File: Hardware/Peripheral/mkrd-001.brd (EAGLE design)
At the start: 25 x 26 mm, 5 parts, among them J1 MKR

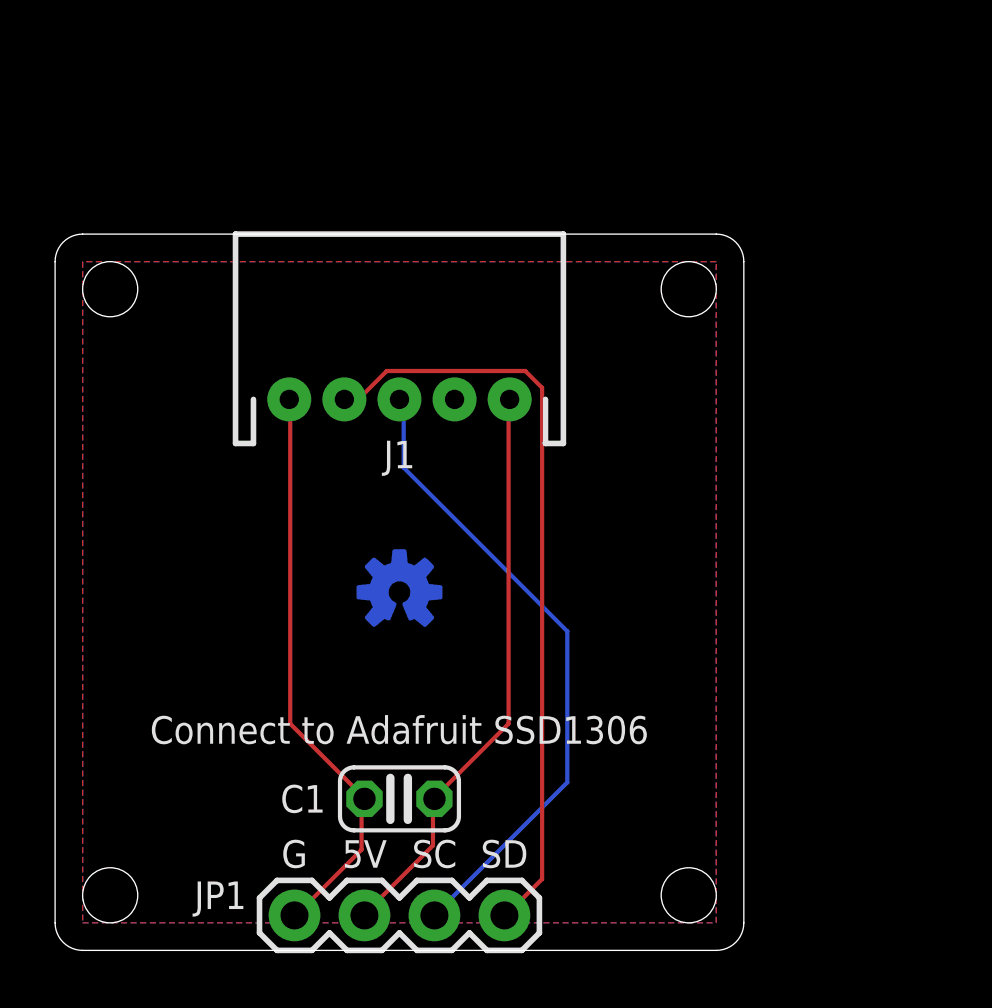
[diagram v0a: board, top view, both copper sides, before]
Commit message: Added new board.
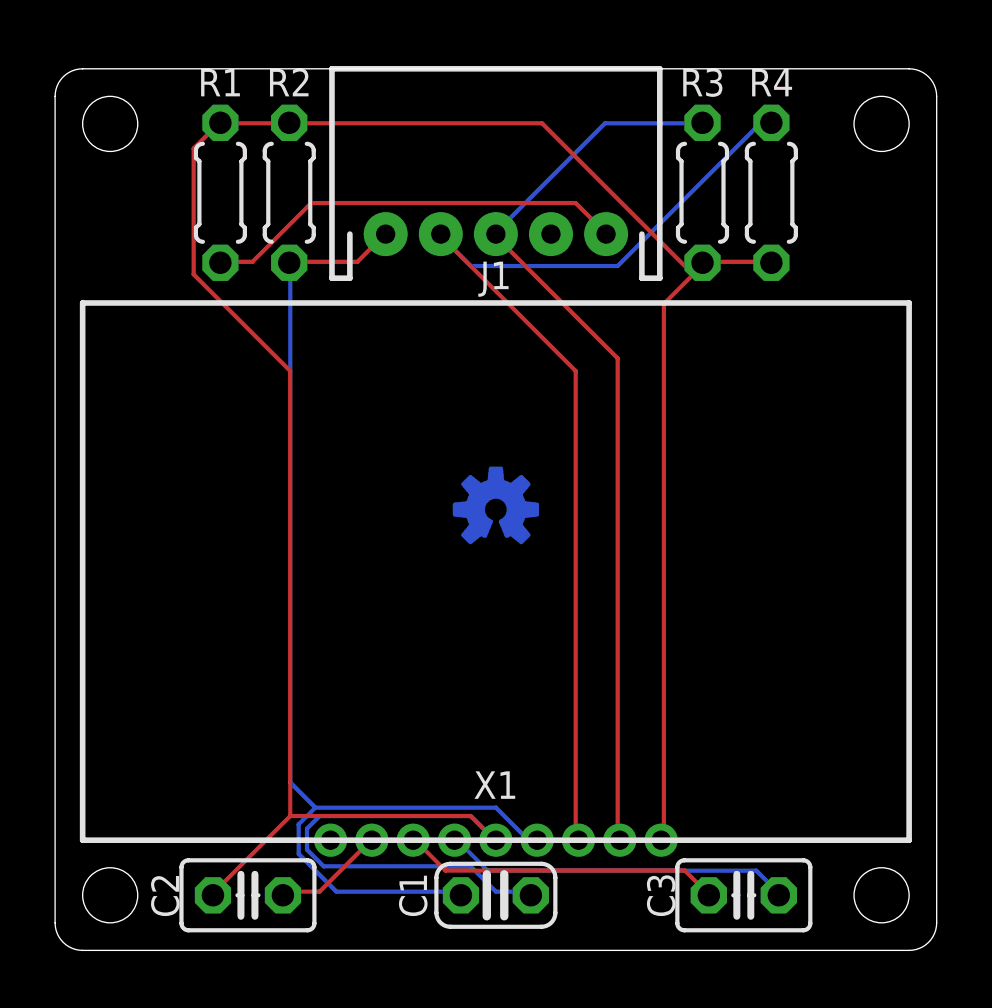
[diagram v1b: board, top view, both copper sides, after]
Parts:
- removed JP1: DISP, SparkFun-Connectors:1X04
- added C2, C3: 1u, rcl:C025-025X050
- added R1: 1.5k, rcl:0204/5
- added R2: 3.3k, rcl:0204/5
- added R3, R4: 10k, rcl:0204/5
- added X1: AQM0802A-RN-GBW, AQM0802A-RN-GBW:AQM0802A-RN-GBW-FOOTPRINT
- C1: value (none) -> 0.1u
- moved J1 6.95 mm to (16.0, 26.0)
- moved C1 4.95 mm to (16.0, 2.00)
- moved LOGO1 4.61 mm to (16.0, 16.0)
- moved U$1 4.61 mm to (16.0, 10.0)
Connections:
- new net 3V3: C1.1, C2.1, R1.2, R2.2, R3.1, R4.1, X1.5, X1.9
- new net N$1: C2.2, X1.2
- new net N$2: C3.2, X1.4
- new net N$3: C3.1, X1.3
- net GND: now also R2.1, X1.6; no longer JP1.1
- net SCL: now also R3.2, X1.8; no longer JP1.3
- net SDA: now also R4.2, X1.7; no longer JP1.4
- net VCC: now also R1.1; no longer C1.1, JP1.2
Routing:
- net 3V3: track 0.00 -> 100.0 mm
- net GND: track 21.0 -> 41.1 mm
- net N$2: track 0.00 -> 12.6 mm
- net N$3: track 0.00 -> 11.6 mm
- net SDA: track 27.6 -> 38.7 mm
- net SCL: track 23.3 -> 33.1 mm
- net VCC: track 20.9 -> 15.4 mm
- net N$1: track 0.00 -> 4.06 mm
- removed copper zone on layer 1, net GND
- removed copper zone on layer 16, net GND
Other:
- board size 25 x 26 mm -> 32 x 32 mm
- board text removed: "5V"
- board text removed: "Connect to Adafruit SSD1306"
- board text removed: "G"
- board text removed: "SC"
- board text removed: "SD"

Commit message: Signal name.
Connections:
- net N$1 renamed LCDVOUT
- net N$2 renamed CAP1P
- net N$3 renamed CAP1N
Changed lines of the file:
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@@
 <wire x1="19.9644" y1="26.0604" x2="20" y2="26" width="0.1524" layer="1"/>
 </signal>
-<signal name="N$2">
+<signal name="CAP1P">
 <contactref element="X1" pad="4"/>
 <contactref element="C3" pad="2"/>
@@
 <wire x1="26.2128" y1="2.1336" x2="26.27" y2="2" width="0.1524" layer="16"/>
 </signal>
-<signal name="N$3">
+<signal name="CAP1N">
 <contactref element="C3" pad="1"/>
 <contactref element="X1" pad="3"/>
@@
 <wire x1="23.622" y1="2.1336" x2="23.73" y2="2" width="0.1524" layer="1"/>
 </signal>
-<signal name="N$1">
+<signal name="LCDVOUT">
 <contactref element="X1" pad="2"/>
 <contactref element="C2" pad="2"/>
